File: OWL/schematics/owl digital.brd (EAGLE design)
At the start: 60 x 57 mm, 59 parts, among them IC1 REG1117, IC3 IS61WV51216BLL-10TLI, U2 WM8731, U4 STM32F405ZGT6

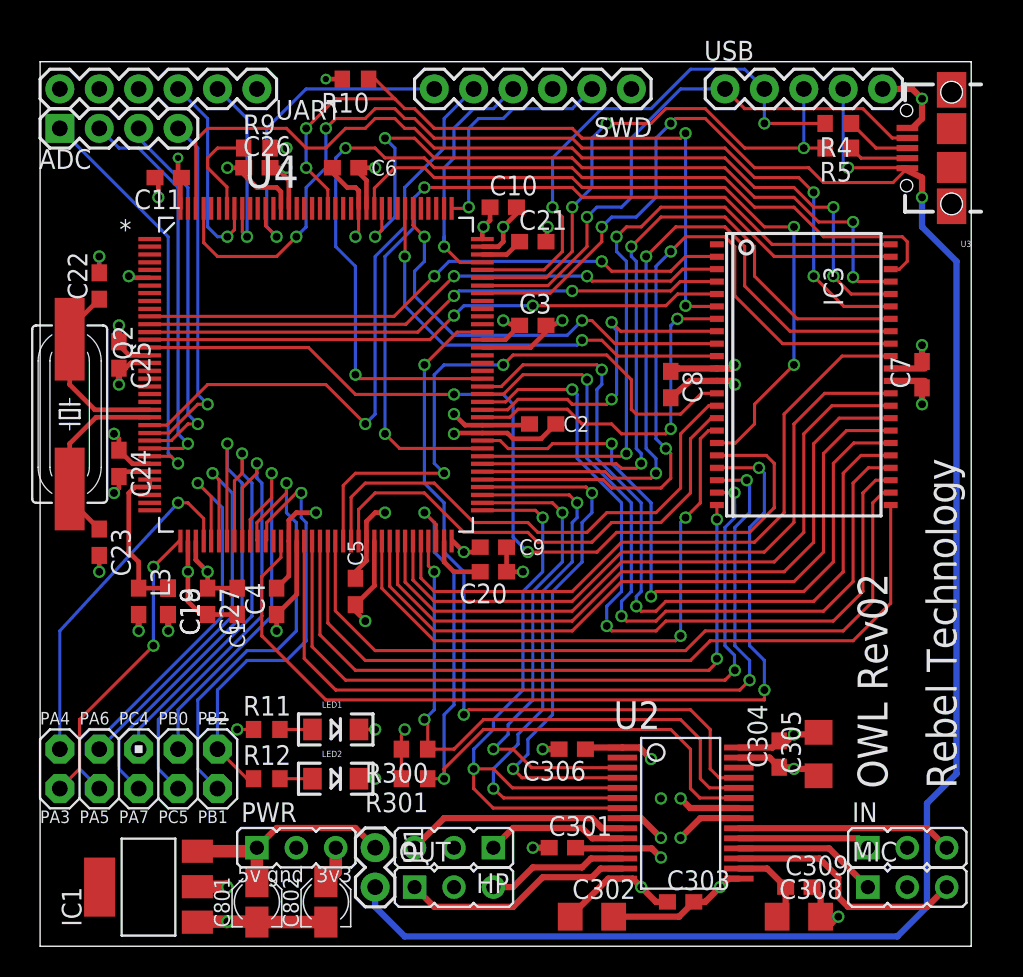
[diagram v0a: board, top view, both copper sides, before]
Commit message: updated usb connector part
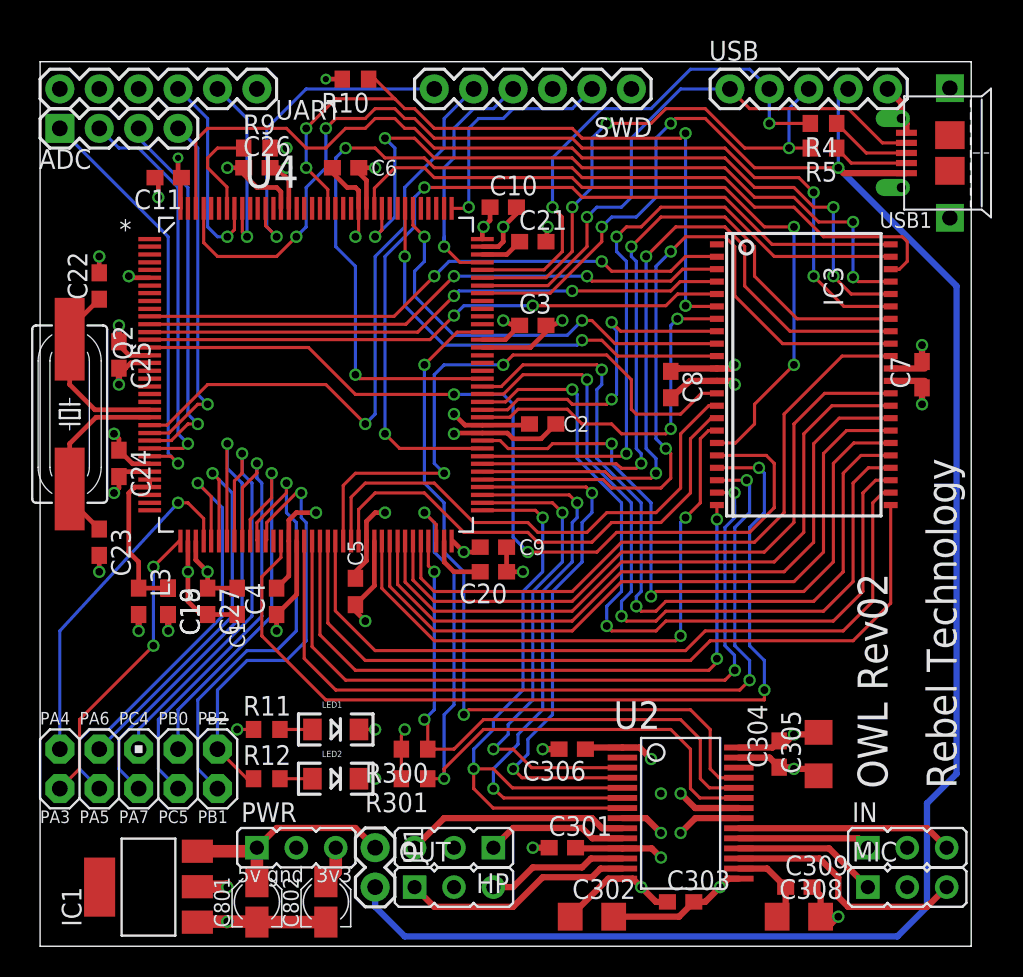
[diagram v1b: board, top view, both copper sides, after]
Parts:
- removed U3: (no value), SparkFun-Connectors:USB-AB-MICRO-SMD
- added USB1: (no value), USB_connector:HRS_ZX62D-AB-5P8_USB
- moved R4 0.95 mm to (50.5, 53.0)
- moved R5 0.95 mm to (50.5, 51.4)
- moved USB 0.32 mm to (44.5, 55.2)
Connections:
- net GND: now also USB1.5, USB1.G, USB1.G2, USB1.G3, USB1.G4; no longer U3.GND
- net N$17: now also USB1.3; no longer U3.D+
- net N$21: now also USB1.2; no longer U3.D-
- net USB_ID: now also USB1.4; no longer U3.ID
- net USB_VBUS: now also USB1.1; no longer U3.VBUS
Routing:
- net USB_VBUS: track 134.7 -> 131.6 mm, vias 4 -> 3
- net GND: track 121.8 -> 119.9 mm, vias 30 -> 29
- net N$17: track 4.26 -> 5.28 mm
- net N$21: track 3.88 -> 4.90 mm
- net USB_DP: track 34.6 -> 33.7 mm
